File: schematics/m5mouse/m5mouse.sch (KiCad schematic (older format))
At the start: 52 parts, among them IC1 LM3940IMP-3.3_NOPB, J1 Conn_01x02, J2 M-BUS, J3 SWD, J6 Conn_01x03, J7 Conn_01x06, J8 Conn_01x06, SW1 SW_SPDT, SW2 SW_Push, U1 TPS562200, U2 STM32F405RGTx, Y1 8MHz, Y2 32.768kHz

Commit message: Put parts
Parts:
- C1, C10, C11, C12, C13, C14, C15, C16, C17, C2, C22, C23, C24, C26, C27, C28, C3, C4, C5, C6, C7, C8, C9: footprint (none) -> Capacitor_SMD:C_0402_1005Metric
- D1, D6, D7: footprint (none) -> LED_SMD:LED_0603_1608Metric
- FB1, R1, R14, R15, R16, R18, R2, R20, R3, R4: footprint (none) -> Resistor_SMD:R_0603_1608Metric
- IC1: footprint SOT230P700X180-4N -> m5mouse:LM3940IMP-3.3NOPB
- J1: footprint (none) -> Connector_JST:JST_EH_B2B-EH-A_1x02_P2.50mm_Vertical
- J2: footprint (none) -> Connector_PinHeader_2.54mm:PinHeader_2x15_P2.54mm_Vertical_SMD
- J3: footprint (none) -> Connector_JST:JST_EH_B6B-EH-A_1x06_P2.50mm_Vertical
- J6: footprint (none) -> Connector_PinHeader_2.54mm:PinHeader_1x03_P2.54mm_Vertical
- J7: footprint (none) -> Connector_PinSocket_2.54mm:PinSocket_1x06_P2.54mm_Vertical
- J8: footprint (none) -> Connector_PinHeader_2.54mm:PinHeader_1x06_P2.54mm_Vertical
- L1: footprint (none) -> Inductor_SMD:L_1008_2520Metric
- R17: value 11k 1% -> 18k 1%; footprint (none) -> Resistor_SMD:R_0603_1608Metric
- R19: value 7.5k 1% -> 10k 1%; footprint (none) -> Resistor_SMD:R_0603_1608Metric
- SW1: footprint (none) -> Button_Switch_THT:SW_E-Switch_EG1224_SPDT_Angled
- SW2: footprint (none) -> Button_Switch_THT:SW_PUSH_6mm
- Y1: footprint (none) -> m5mouse:CSTNE8M00G55Z000R0
- Y2: footprint (none) -> m5mouse:XRCGB32M768F2N10R0; symbol Device:Crystal -> Device:Crystal_GND24
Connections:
- net GND: now also Y2.2, Y2.4
- net GPIO1: now also U2.33 (PB12); no longer U2.2 (PC13)
- net GPIO10: now also U2.34 (PB13); no longer U2.52 (PC11)
- net GPIO11: now reaches U2.20 (PA4)
- net GPIO11: now also U2.52 (PC11)
- net SPI1_SCK: now reaches U2.21 (PA5)
- net at C9.1, U2.4 (PC15): now also Y2.3; no longer Y2.2
- net SPI1_CS: now reaches U2.53 (PC12)
- net SPI1_MISO: now reaches U2.56 (PB4)
- net SPI1_MOSI: now reaches U2.57 (PB5)
- no-connect marks 44 -> 38
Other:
- note added: "8.4V to 3V"
- note removed: "7.4V to 3V"
- moved on the sheet: C26, C27, C9, IC1, J1, J2, R17, R19, SW1

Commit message: Adjust parts positions
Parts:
- J1: footprint Connector_JST:JST_EH_B2B-EH-A_1x02_P2.50mm_Vertical -> Connector_JST:JST_PH_B2B-PH-K_1x02_P2.00mm_Vertical
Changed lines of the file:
@@
 F 0 "J1" H 1430 4642 50  0000 L CNN
 F 1 "Conn_01x02" H 1430 4551 50  0000 L CNN
-F 2 "Connector_JST:JST_EH_B2B-EH-A_1x02_P2.50mm_Vertical" H 1350 4650 50  0001 C CNN
+F 2 "Connector_JST:JST_PH_B2B-PH-K_1x02_P2.00mm_Vertical" H 1350 4650 50  0001 C CNN
 F 3 "~" H 1350 4650 50  0001 C CNN
 	1    1350 4650

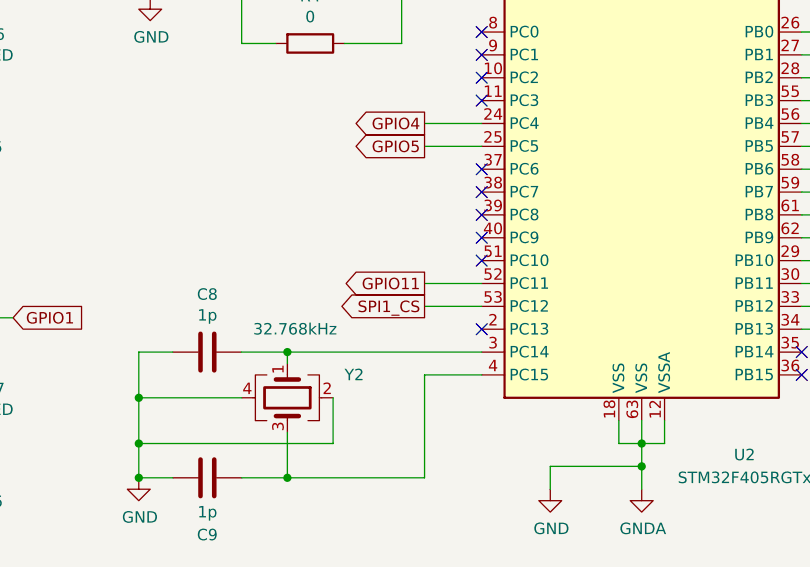
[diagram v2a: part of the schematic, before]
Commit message: Draw pattern
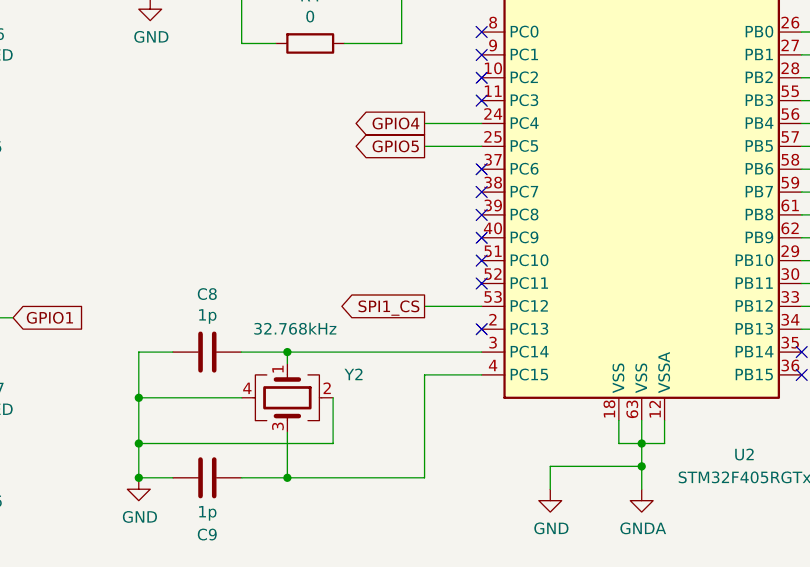
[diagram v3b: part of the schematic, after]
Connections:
- net GPIO11: no longer U2.52 (PC11)
- no-connect marks 38 -> 39
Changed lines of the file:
@@
 GPIO11
 NoConn ~ 13000 5300
-Text GLabel 11350 6600 0    50   Output ~ 0
-GPIO11
-Wire Wire Line
-	11350 6600 11600 6600
 Text GLabel 11350 6700 0    50   Output ~ 0
 SPI1_CS
@@
 Wire Wire Line
 	14200 3600 15000 3600
+NoConn ~ 11600 6600
 $EndSCHEMATC
